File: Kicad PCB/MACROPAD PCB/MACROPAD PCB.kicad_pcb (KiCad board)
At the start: 2 copper layers, 85.7 x 111.9 mm, 33 parts, among them SW1 SW_Push, SW10 SW_Push, SW11 SW_Push, SW12 SW_Push, SW13 SW_Push, SW14 SW_Push, SW15 SW_Push, SW16 SW_Push, SW2 SW_Push, SW3 SW_Push, SW4 SW_Push, SW5 SW_Push, SW6 SW_Push, SW7 SW_Push, SW8 SW_Push, SW9 SW_Push, U1 RP2040-ZERO

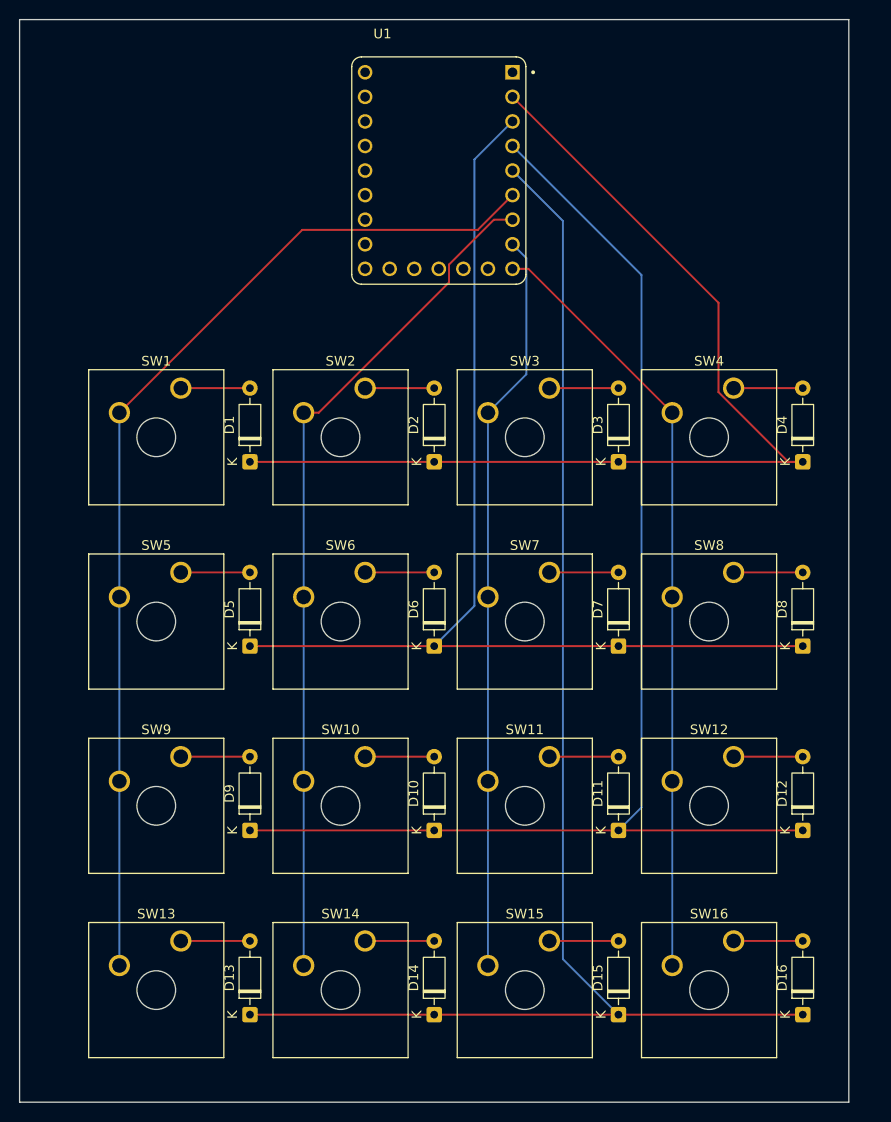
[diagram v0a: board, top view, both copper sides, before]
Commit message: PCB
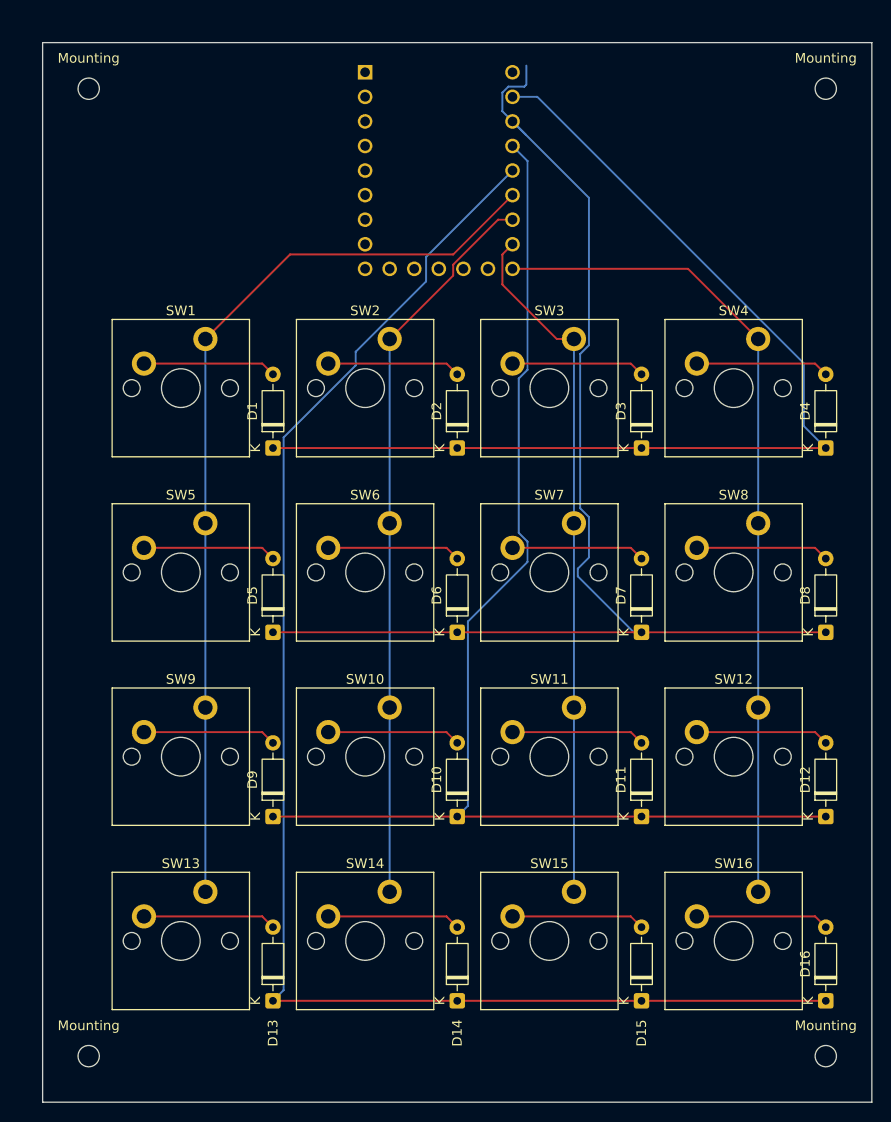
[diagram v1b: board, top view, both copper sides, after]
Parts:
- added Mounting: MountingHole_2.2mm_M2, MountingHole:MountingHole_2.2mm_M2, F.Cu at (147.6, 33.3)
- added Mounting: MountingHole_2.2mm_M2, MountingHole:MountingHole_2.2mm_M2, F.Cu at (71.4, 33.3)
- added Mounting: MountingHole_2.2mm_M2, MountingHole:MountingHole_2.2mm_M2, F.Cu at (147.6, 133.3)
- added Mounting: MountingHole_2.2mm_M2, MountingHole:MountingHole_2.2mm_M2, F.Cu at (71.4, 133.3)
- SW1, SW10, SW11, SW12, SW13, SW14, SW15, SW16, SW2, SW3, SW4, SW5, SW6, SW7, SW8, SW9: footprint Button_Switch_Keyboard:SW_Cherry_MX_1.00u_Plate -> PCM_Switch_Keyboard_Cherry_MX:SW_Cherry_MX_PCB_1.00u
- U1: moved to B.Cu
- moved D11 2.78 mm to (128.6, 108.6)
- moved D7 2.78 mm to (128.6, 89.5)
- moved D15 2.78 mm to (128.6, 127.6)
- moved D3 2.78 mm to (128.6, 70.5)
- moved D10 2.78 mm to (109.5, 108.6)
- moved D12 2.78 mm to (147.6, 108.6)
- moved D5 2.78 mm to (90.5, 89.5)
- moved D6 2.78 mm to (109.5, 89.5)
- moved D8 2.78 mm to (147.6, 89.5)
- moved D9 2.78 mm to (90.5, 108.6)
- moved D1 2.78 mm to (90.5, 70.5)
- moved D13 2.78 mm to (90.5, 127.6)
- moved D14 2.78 mm to (109.5, 127.6)
- moved D16 2.78 mm to (147.6, 127.6)
- moved D2 2.78 mm to (109.5, 70.5)
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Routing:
- net ROW1: track 114.7 -> 127.8 mm
- net COL1: track 88.1 -> 75.6 mm
- net COL0: track 107.1 -> 95.1 mm
- net Net-(D7-A): track 7.14 -> 13.8 mm
- net Net-(D8-A): track 7.14 -> 13.8 mm
- net Net-(D3-A): track 7.14 -> 13.8 mm
- net Net-(D6-A): track 7.14 -> 13.8 mm
- net Net-(D5-A): track 7.14 -> 13.8 mm
- net Net-(D4-A): track 7.14 -> 13.8 mm
- net Net-(D15-A): track 7.14 -> 13.8 mm
- net Net-(D11-A): track 7.14 -> 13.8 mm
- net Net-(D2-A): track 7.14 -> 13.8 mm
- net Net-(D16-A): track 7.14 -> 13.8 mm
- net Net-(D12-A): track 7.14 -> 13.8 mm
- net Net-(D1-A): track 7.14 -> 13.8 mm
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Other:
- board size 85.7 x 111.9 mm -> 85.7 x 109.5 mm
